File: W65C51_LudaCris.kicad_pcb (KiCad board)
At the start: 4 copper layers, 105.1 x 79.7 mm, 31 parts, among them U1 W65C51NxP, U10 74HC283, U11 74HC191, U2 74HC138, U3 74HC573, U4 ATF22V10, U5 ATF22V10, U6 74HC191, U7 74HC191, U8 74HC191, U9 74HC191

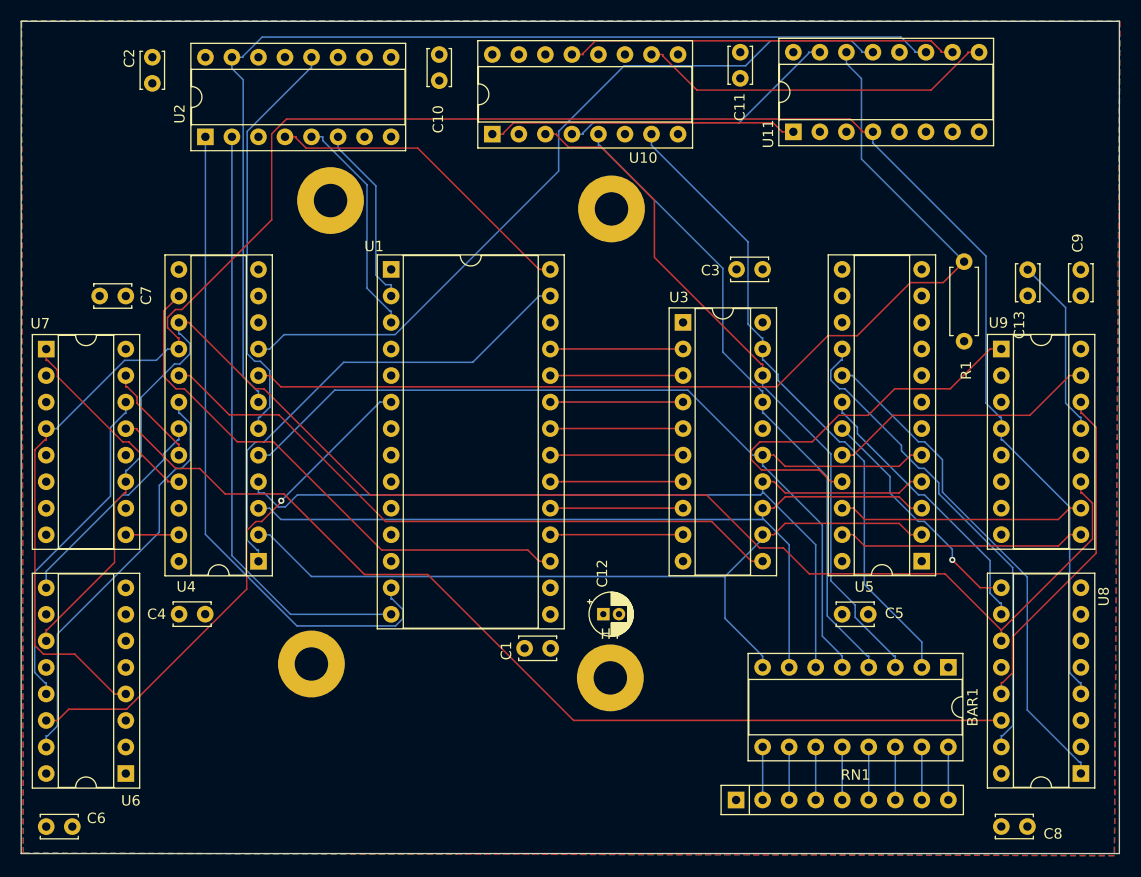
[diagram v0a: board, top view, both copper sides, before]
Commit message: pcb
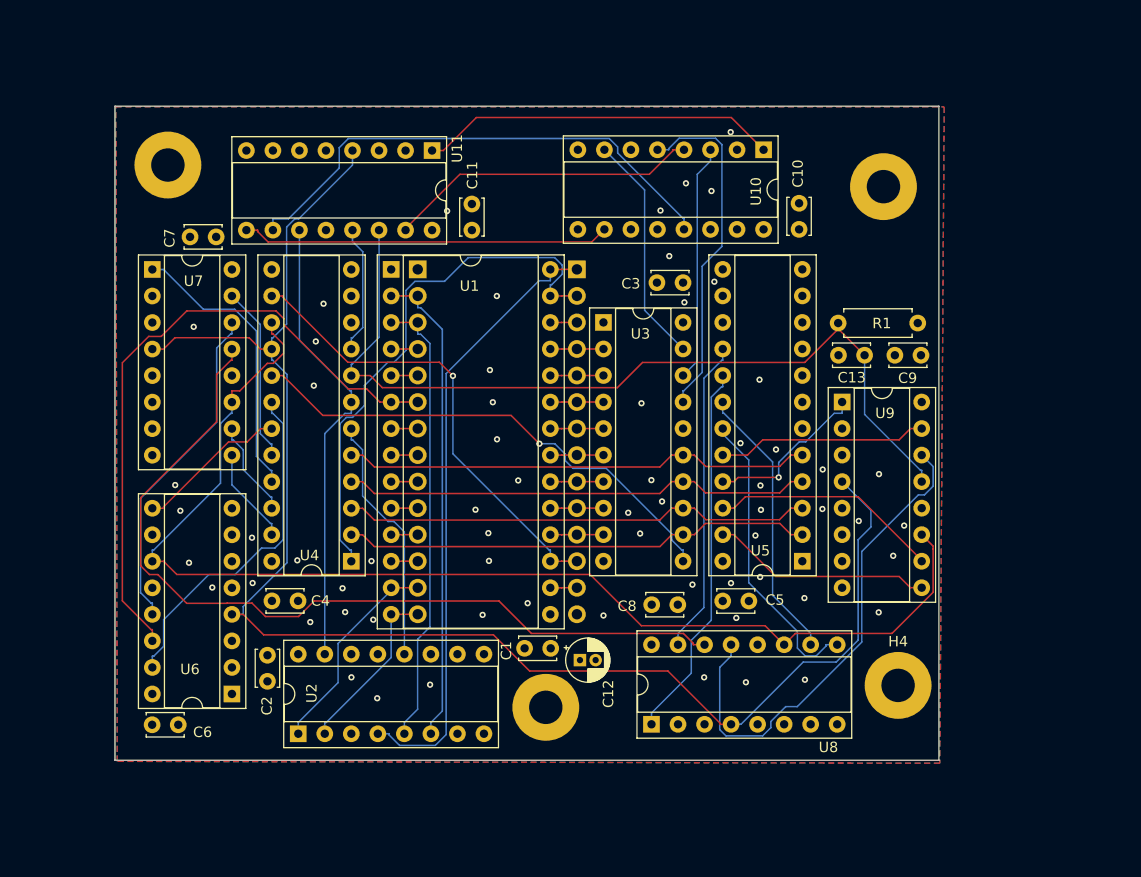
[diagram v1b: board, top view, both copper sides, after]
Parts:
- removed BAR1: LED-Array-8, Package_DIP:DIP-16_W7.62mm_Socket
- removed RN1: 220, Resistor_THT:R_Array_SIP9
- added J1: Conn_01x14, Connector_PinHeader_2.54mm:PinHeader_1x14_P2.54mm_Vertical, B.Cu at (133.5, 73.7)
- added J2: Conn_01x14, Connector_PinHeader_2.54mm:PinHeader_1x14_P2.54mm_Vertical, B.Cu at (148.8, 73.7)
- moved C2 60.8 mm to (119.1, 113.1), turned to 90 degrees
- moved U2 57.8 mm to (122.1, 118.1)
- moved U8 41.4 mm to (155.9, 117.2), turned to 90 degrees
- moved C8 39.6 mm to (155.9, 105.8)
- moved C10 38.3 mm to (170.0, 69.8), turned to 90 degrees
- moved U11 34.6 mm to (134.9, 62.3), turned to -90 degrees
- moved C11 30.8 mm to (138.7, 69.9), turned to 90 degrees
- moved H4 27.6 mm to (179.5, 113.5)
- moved H1 26.1 mm to (178.1, 65.8)
- moved U10 26.0 mm to (166.6, 62.2), turned to -90 degrees
- moved H2 22.8 mm to (145.8, 115.6)
- moved C13 17.6 mm to (176.3, 81.9), turned to 180 degrees
- moved C9 16.3 mm to (181.7, 81.9), turned to 180 degrees
- moved U9 16.1 mm to (174.1, 86.4)
- moved H3 15.9 mm to (109.6, 63.7)
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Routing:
- net /~{TX_COMPLETE}: track 73.8 -> 12.3 mm
- net /~{TX_START}: track 102.1 -> 44.1 mm
- net /CR3: track 93.2 -> 45.0 mm
- net /~{CTEN}: track 194.5 -> 148.3 mm
- net /CR6: track 67.6 -> 22.7 mm
- net /RS0: track 64.4 -> 20.2 mm
- net /CR2: track 86.5 -> 45.0 mm
- net /RS1: track 57.7 -> 16.7 mm
- net /CR7: track 62.2 -> 22.2 mm
- net /~{BAUD_CLK}: track 121.5 -> 83.2 mm
- net /CR1: track 81.2 -> 45.0 mm
- net /CR0: track 78.1 -> 45.0 mm
- net /~{BAUD_LOAD}: track 147.6 -> 115.6 mm
- net /CR5: track 62.1 -> 33.2 mm
- net /R~{W}: track 30.7 -> 59.3 mm
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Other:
- board size 105.1 x 79.7 mm -> 78.9 x 62.6 mm
